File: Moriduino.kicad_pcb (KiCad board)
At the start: 2 copper layers, 68.6 x 53.3 mm, 41 parts, among them CN1 CON_USB-C-16, CN2 CON_AVRISP, J1 USB_B, J2 Barrel_Jack_Switch, P1 Power, P2 Analog, P3 Digital, P4 Digital, P5 CONN_01X01, P6 CONN_01X01, P7 CONN_01X01, Q1 FDN340P, U1 AP1117-50, U2 LMV358, U3 IC_FT232RQ, U4 ATmega328P-PU, U5 LDO_5p_NJM2865, Y1 16MHz

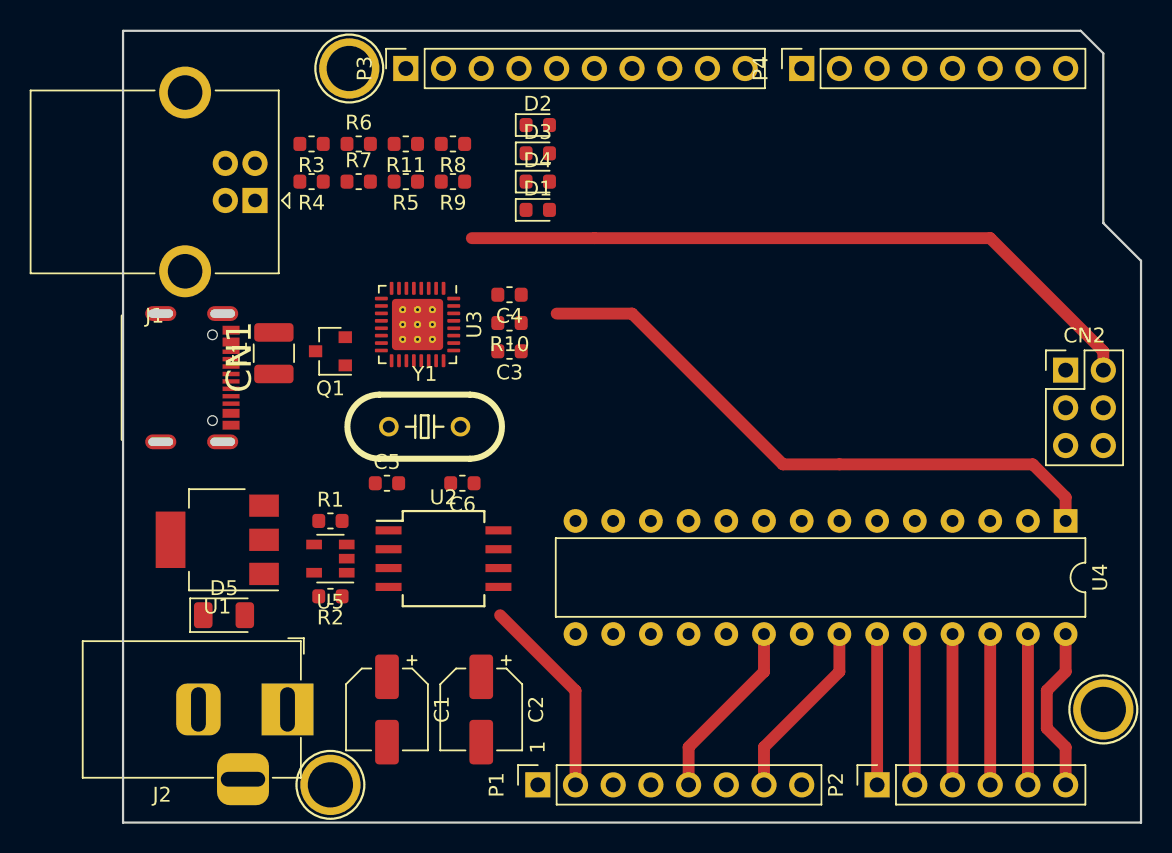
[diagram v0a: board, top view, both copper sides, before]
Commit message: 配線を少し進めた
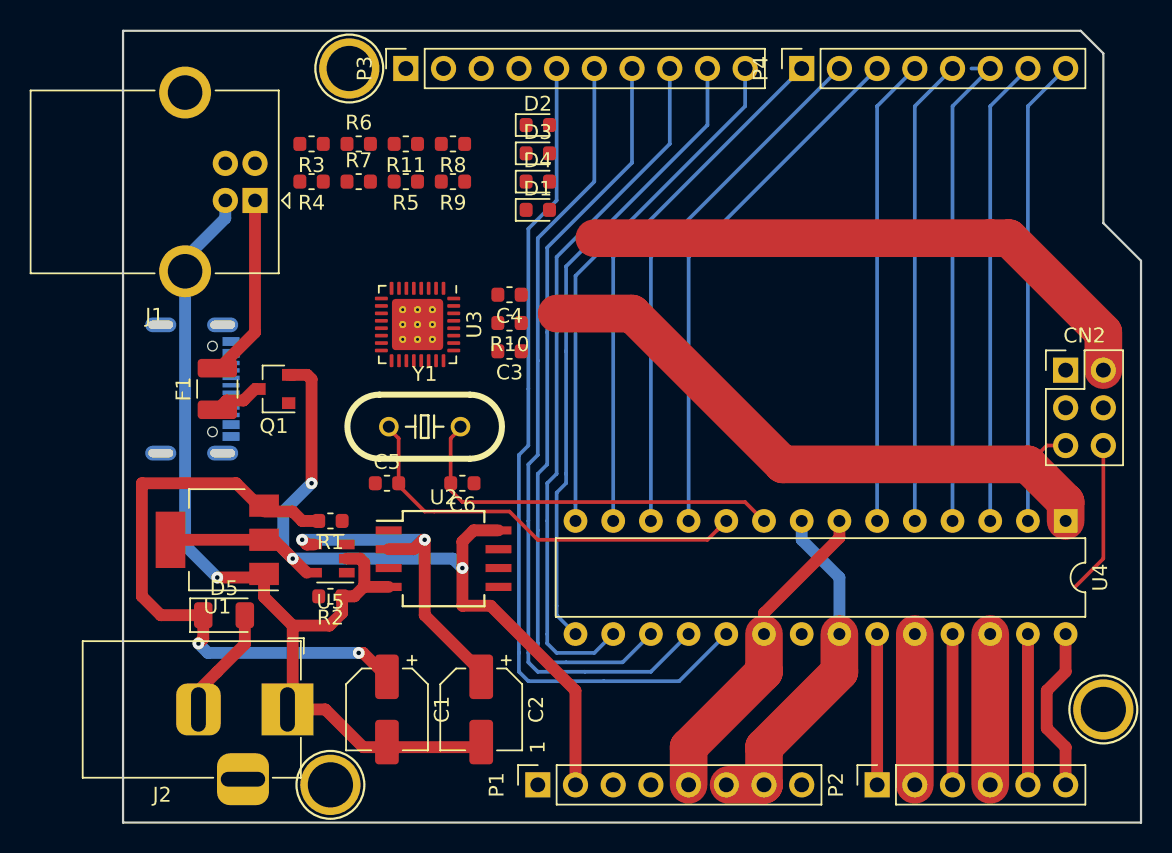
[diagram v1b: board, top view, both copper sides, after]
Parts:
- CN1: moved to B.Cu
- moved Q1 4.58 mm to (121.2, 97.2)
- moved F1 4.51 mm to (117.3, 97.2)
- moved CN1 0.76 mm to (117.3, 97.2), turned to 90 degrees
- turned R1 to 180 degrees
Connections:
- U1 pad 1: Net-(U1-Pad1) -> GND
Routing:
- net GND: track 12.3 -> 100.2 mm, vias 0 -> 1
- net /D13: track 0.00 -> 57.2 mm
- net /D12: track 0.00 -> 54.0 mm
- net /D11: track 0.00 -> 50.7 mm
- net +5V: track 72.8 -> 120.8 mm, vias 0 -> 3
- net /D10: track 0.00 -> 47.4 mm
- net /D9: track 0.00 -> 43.5 mm
- net /VIN: track 0.00 -> 40.4 mm, vias 0 -> 2
- net /D6: track 0.00 -> 35.7 mm
- net /D7: track 0.00 -> 35.7 mm
- net /D5: track 0.00 -> 35.7 mm
- net /D8: track 0.00 -> 35.2 mm
- net /D2: track 0.00 -> 32.8 mm
- net /D4: track 0.00 -> 31.5 mm
- net /D3: track 0.00 -> 31.5 mm
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
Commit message: 一通り完成
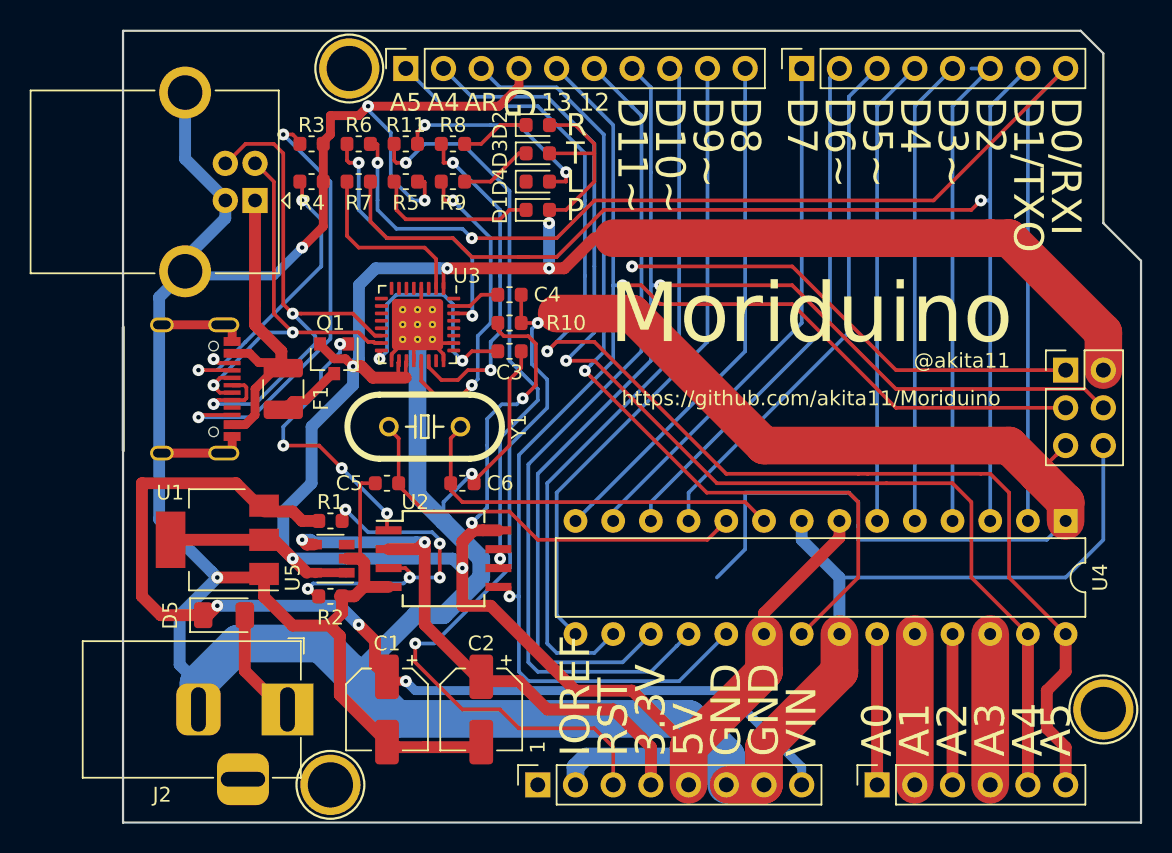
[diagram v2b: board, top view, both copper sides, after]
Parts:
- CN1: moved to F.Cu
- moved Q1 4.54 mm to (125.2, 95.1), turned to 270 degrees
- moved F1 4.45 mm to (121.8, 97.2)
- moved CN1 0.08 mm to (117.3, 97.2), turned to 270 degrees
- turned R11 to 0 degrees
- turned R6 to 180 degrees
- turned R7 to 180 degrees
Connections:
- D2 pad 2: Net-(D2-Pad2) -> +5V
- D3 pad 2: Net-(D3-Pad2) -> +5V
- J2 pad 1: GND -> Net-(D5-Pad2)
- J2 pad 2: Net-(D5-Pad2) -> GND
- U3 pad 33: (no net) -> GND
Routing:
- net GND: track 100.2 -> 287.8 mm, vias 1 -> 5
- net +5V: track 120.8 -> 205.3 mm, vias 3 -> 8
- net /RST: track 43.9 -> 125.7 mm, vias 0 -> 2
- net /A5: track 11.2 -> 86.7 mm, vias 0 -> 1
- net /A4: track 10.2 -> 79.5 mm, vias 0 -> 1
- net /AREF: track 0.00 -> 59.1 mm, vias 0 -> 1
- net /D0: track 31.5 -> 88.3 mm, vias 0 -> 2
- net /D1: track 31.5 -> 79.2 mm, vias 0 -> 1
- net /D13: track 57.2 -> 96.2 mm, vias 0 -> 2
- net Net-(R11-Pad1): track 0.00 -> 38.7 mm, vias 0 -> 2
- net /USB_DP: track 0.00 -> 38.3 mm, vias 0 -> 2
- net /D12: track 54.0 -> 89.4 mm, vias 0 -> 1
- net /D11: track 50.7 -> 85.6 mm, vias 0 -> 1
- net /VIN: track 40.4 -> 72.2 mm, vias 2 -> 3
- net Net-(CN1-PadB5): track 0.00 -> 30.0 mm, vias 0 -> 2
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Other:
- board text added: "12"
- board text added: "13"
- board text added: "3.3V"
- board text added: "5V"
- board text added: "@akita11"
- board text added: "A0"
- board text added: "A1"
- board text added: "A2"
- board text added: "A3"
- board text added: "A4"
- board text added: "A5"
- board text added: "AR"
- board text added: "D0/RXI"
- board text added: "D1/TXO"
- board text added: "D10~~"
- board text added: "D11~~"
- board text added: "D2"
- board text added: "D3~~"
- board text added: "D4"
- board text added: "D5~~"
- board text added: "D6~~"
- board text added: "D7"
- board text added: "D8"
- board text added: "D9~~"
- board text added: "G"
- board text added: "GND"
- board text added: "IOREF"
- board text added: "L"
- board text added: "Moriduino"
- board text added: "P"
- board text added: "R"
- board text added: "RST"
- board text added: "T"
- board text added: "VIN"
- board text added: "https://github.com/akita11/Moriduino"

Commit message: 配線ミスを修正しベタGNDを追加
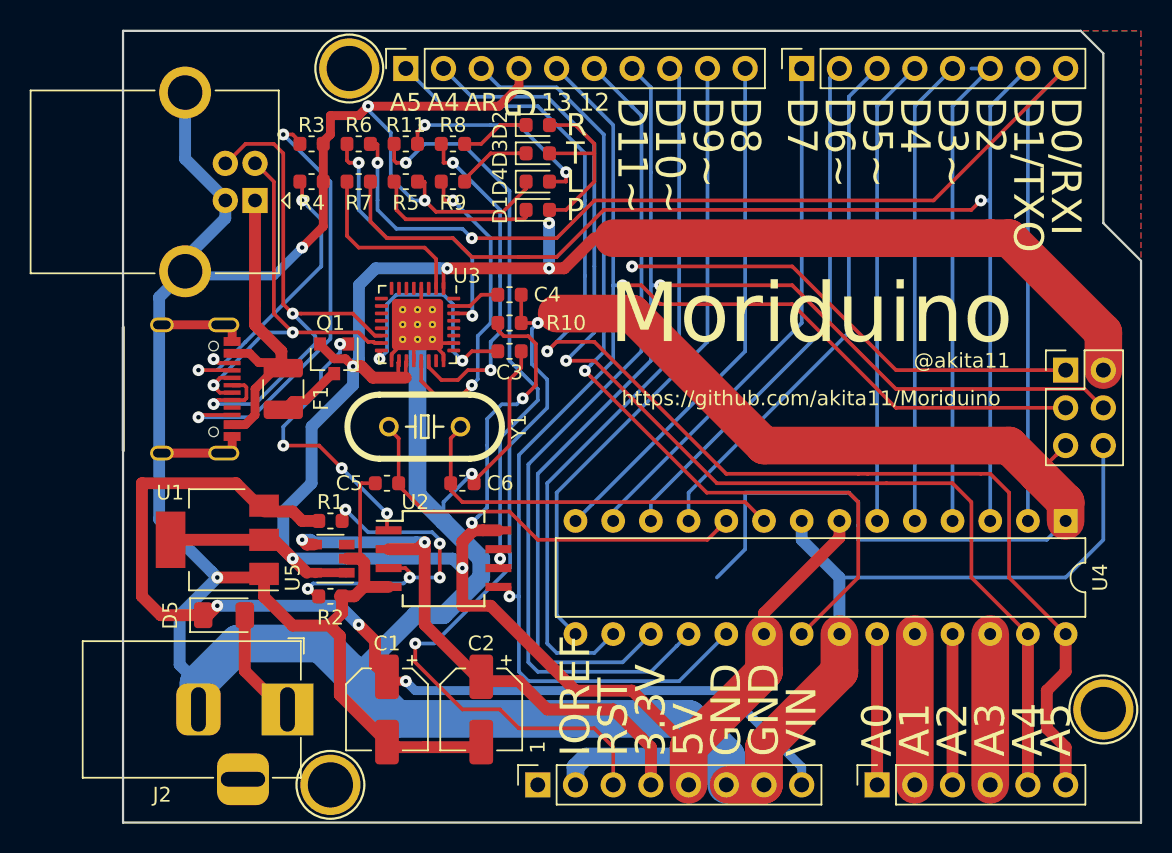
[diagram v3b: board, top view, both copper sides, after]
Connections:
- D4 pad 1: Net-(D4-Pad1) -> GND
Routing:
- net GND: track 287.8 -> 296.1 mm
- added copper zone on B.Cu, net GND
- added copper zone on F.Cu, net GND

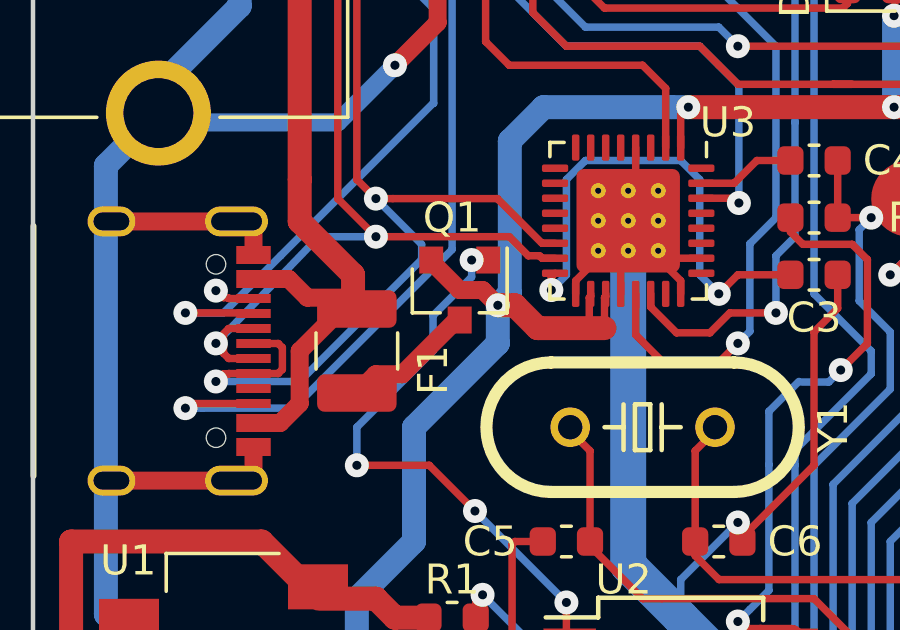
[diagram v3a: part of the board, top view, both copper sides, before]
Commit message: pMOSの向きが逆だったのを修正
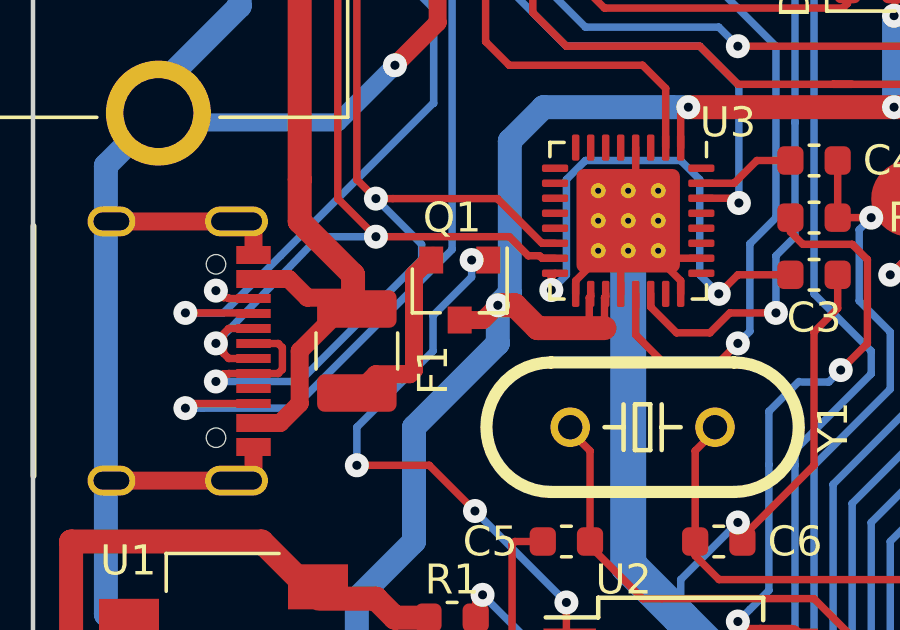
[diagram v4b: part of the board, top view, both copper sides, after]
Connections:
- Q1 pad 2: +5V -> Net-(F1-Pad1)
- Q1 pad 3: Net-(F1-Pad1) -> +5V
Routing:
- net Net-(F1-Pad1): track 4.81 -> 6.85 mm
- net +5V: track 205.3 -> 203.9 mm
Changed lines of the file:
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@@
     (thickness 1.6)
     (drawings 47)
-    (tracks 722)
+    (tracks 724)
     (zones 0)
     (modules 41)
@@
   )
   (setup
-    (last_trace_width 0.25)
+    (last_trace_width 0.6)
     (user_trace_width 0.4)
     (user_trace_width 0.6)
@@
     )
     (pad 3 smd rect (at 1 0 270) (size 0.9 0.8) (layers F.Cu F.Paste F.Mask)
+      (net 1 +5V))
+    (pad 2 smd rect (at -1 0.95 270) (size 0.9 0.8) (layers F.Cu F.Paste F.Mask)
       (net 17 "Net-(F1-Pad1)"))
-    (pad 2 smd rect (at -1 0.95 270) (size 0.9 0.8) (layers F.Cu F.Paste F.Mask)
-      (net 1 +5V))
     (pad 1 smd rect (at -1 -0.95 270) (size 0.9 0.8) (layers F.Cu F.Paste F.Mask)
       (net 18 "Net-(Q1-Pad1)"))
@@
   (via (at 139.7 89.027) (size 0.8) (drill 0.3) (layers F.Cu B.Cu) (net 1))
   (segment (start 126.603 95.52) (end 126.492 95.631) (width 0.6) (layer F.Cu) (net 1))
-  (segment (start 124.272 94.173) (end 125.222 95.123) (width 0.6) (layer F.Cu) (net 1))
-  (segment (start 124.272 94.123) (end 124.272 94.173) (width 0.6) (layer F.Cu) (net 1))
-  (segment (start 125.984 95.123) (end 126.492 95.631) (width 0.6) (layer F.Cu) (net 1))
-  (segment (start 125.222 95.123) (end 125.984 95.123) (width 0.6) (layer F.Cu) (net 1))
+  (segment (start 124.272 94.123) (end 124.272 94.173) (width 0.6) (layer F.Cu) (net 17))
   (segment (start 128.016 89.027) (end 132.276315 89.027) (width 0.8) (layer B.Cu) (net 1))
   (segment (start 126.492 95.631) (end 126.891999 95.231001) (width 0.8) (layer B.Cu) (net 1))
@@
   (segment (start 123.698 99.695) (end 123.698 103.505) (width 0.8) (layer B.Cu) (net 1))
   (segment (start 126.492 96.901) (end 123.698 99.695) (width 0.8) (layer B.Cu) (net 1))
+  (segment (start 126 96.123) (end 126.492 95.631) (width 0.6) (layer F.Cu) (net 1))
+  (segment (start 125.222 96.123) (end 126 96.123) (width 0.6) (layer F.Cu) (net 1))
   (segment (start 120.498 111.165) (end 122.428 113.095) (width 0.8) (layer F.Cu) (net 2))
   (segment (start 120.498 109.615) (end 120.498 111.165) (width 0.8) (layer F.Cu) (net 2))
@@
   (segment (start 122.418 97.93) (end 123.304 97.93) (width 0.6) (layer F.Cu) (net 17))
   (segment (start 121.793 98.555) (end 122.418 97.93) (width 0.6) (layer F.Cu) (net 17))
-  (segment (start 123.304 97.93) (end 125.095 96.139) (width 0.6) (layer F.Cu) (net 17))
+  (segment (start 123.304 97.93) (end 123.558 97.93) (width 0.6) (layer F.Cu) (net 17))
+  (segment (start 123.558 97.93) (end 123.698 97.79) (width 0.6) (layer F.Cu) (net 17))
+  (segment (start 123.698 97.79) (end 123.698 94.615) (width 0.6) (layer F.Cu) (net 17))
+  (segment (start 123.698 94.615) (end 124.333 93.98) (width 0.6) (layer F.Cu) (net 17))
   (via (at 125.73 102.489) (size 0.8) (drill 0.3) (layers F.Cu B.Cu) (net 18))
   (segment (start 125.73 102.489) (end 128.778 105.537) (width 0.25) (layer B.Cu) (net 18))
